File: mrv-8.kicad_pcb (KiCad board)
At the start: 2 copper layers, 68.6 x 24.1 mm, 20 parts, among them J1 Conn_02x05_Odd_Even, U1 MCP23008-xSO, U2 ULN2803A

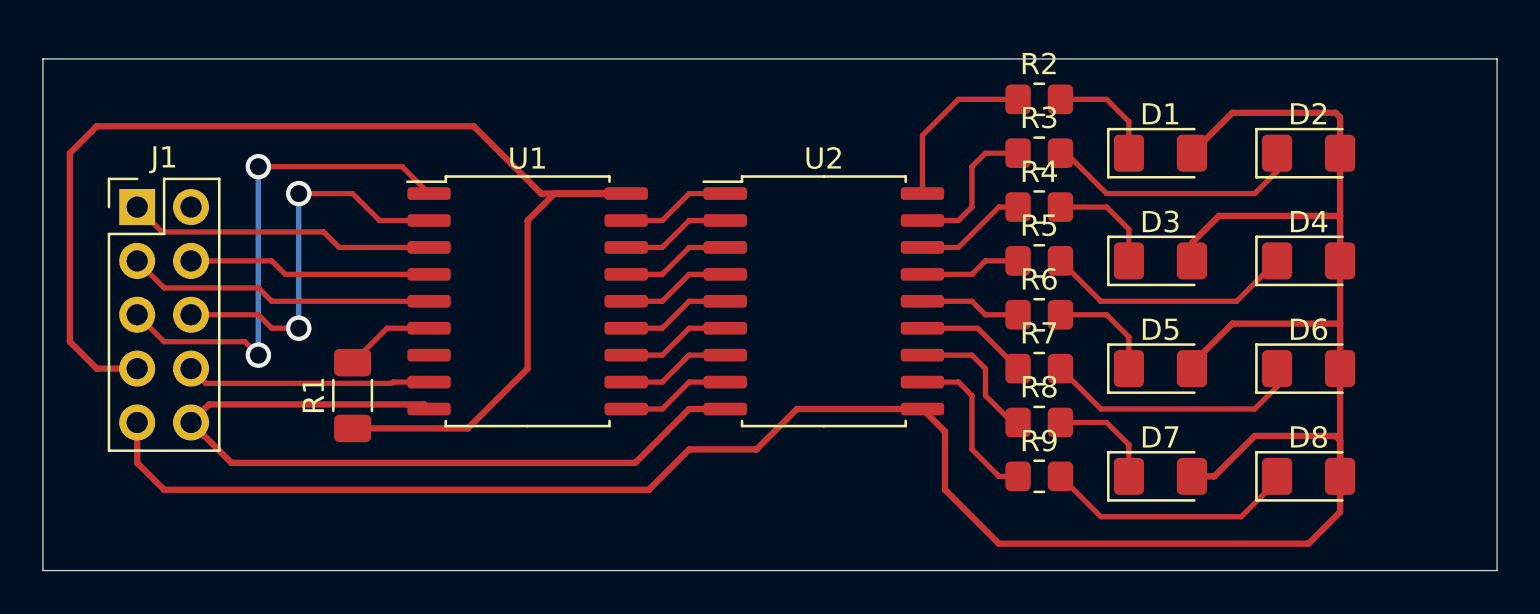
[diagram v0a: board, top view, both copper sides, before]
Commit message: edit pcb mrv-8
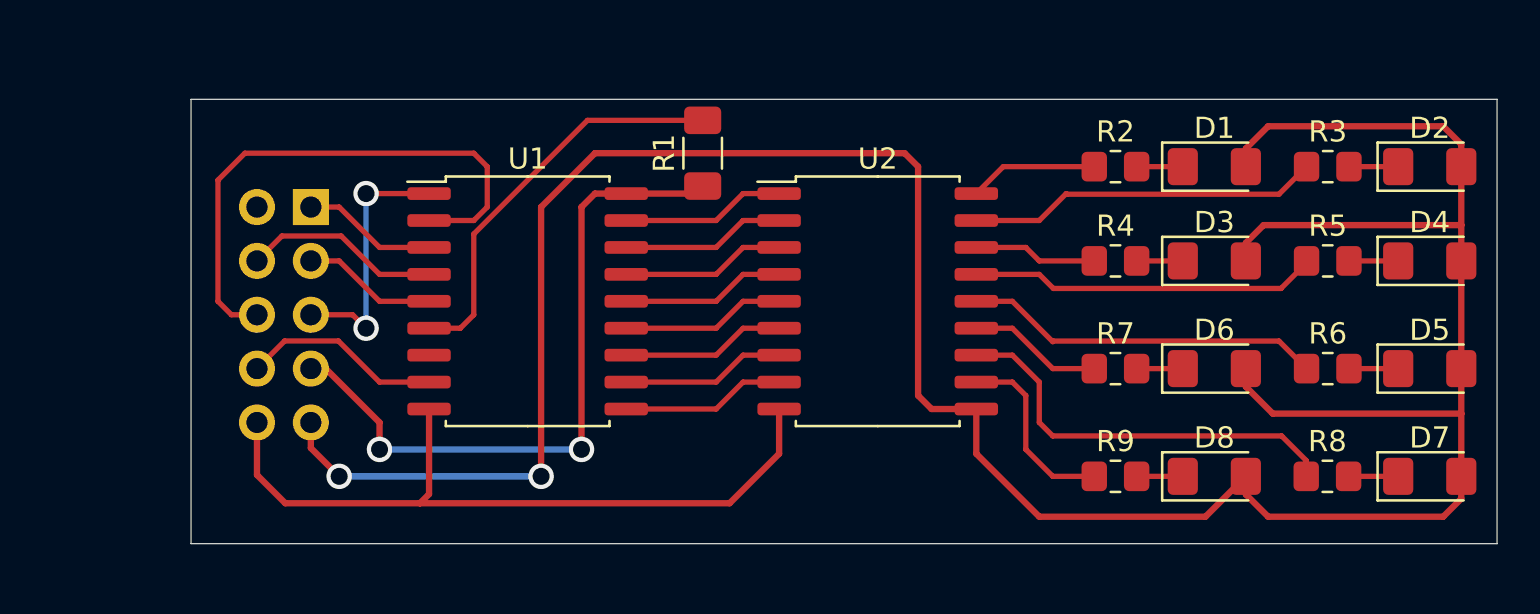
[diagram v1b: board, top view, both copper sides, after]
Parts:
- J1: footprint Connector_PinHeader_2.54mm:PinHeader_2x05_P2.54mm_Vertical -> Connector_PinHeader_2.54mm:PinHeader_2x05_P2.54mm_Horizontal; moved to B.Cu
- moved R1 20.1 mm to (167.0, 74.3)
- moved R6 13.8 mm to (196.5, 84.5)
- moved R8 13.8 mm to (196.5, 89.5)
- moved R3 13.6 mm to (196.5, 74.9)
- moved R5 13.6 mm to (196.5, 79.4)
- moved D5 12.7 mm to (201.3, 84.5)
- moved D7 12.7 mm to (201.3, 89.5)
- moved J1 8.19 mm to (148.5, 76.8), turned to 180 degrees
- moved D2 5.75 mm to (201.3, 74.9)
- moved D4 5.71 mm to (201.3, 79.4)
- moved R2 4.79 mm to (186.5, 74.9)
- moved D6 4.45 mm to (191.1, 84.5)
- moved D8 4.45 mm to (191.1, 89.5)
- moved R4 4.40 mm to (186.5, 79.4)
- moved R7 3.59 mm to (186.5, 84.5)
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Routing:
- net +3V3: track 62.3 -> 32.6 mm, vias 0 -> 2
- net +5VD: track 118.0 -> 138.3 mm, vias 0 -> 2
- net Net-(R1-Pad2): track 4.28 -> 19.2 mm
- net Net-(R8-Pad1): track 6.57 -> 19.5 mm
- net Net-(R6-Pad1): track 4.77 -> 16.9 mm
- net Net-(J1-Pad5): track 24.0 -> 12.2 mm
- net Net-(R5-Pad1): track 4.77 -> 16.4 mm
- net Net-(D6-Pad1): track 12.3 -> 2.18 mm
- net Net-(D2-Pad1): track 12.3 -> 2.32 mm
- net Net-(D8-Pad1): track 11.9 -> 2.18 mm
- net Net-(R3-Pad1): track 6.94 -> 16.7 mm
- net Net-(D4-Pad1): track 11.8 -> 2.32 mm
- net Net-(J1-Pad3): track 14.6 -> 6.36 mm
- net Net-(J1-Pad1): track 14.6 -> 6.36 mm
- net Net-(J1-Pad6): track 18.4 -> 26.2 mm, vias 2 -> 0
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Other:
- board size 68.6 x 24.1 mm -> 61.6 x 21 mm
